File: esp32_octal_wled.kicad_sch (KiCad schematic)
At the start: 54 parts, among them J1 LED1, J11 I2C_Display, J12 ATX-24, J13 LED1, J14 LED1, J15 LED1, J16 LED1, J2 LED1, J3 PROG, J4 LED1, J5 EXT2, J6 LED1, J7 LED1, J8 CPU12V, Q2 BC847, SW1 ON 485 OFF, SW2 RESET, SW4 PROG, U1 AMS1117-3.3, U2 ESP32-WROOM-E, U3 74AHCT125, U4 74AHCT125, U5 MAX3485

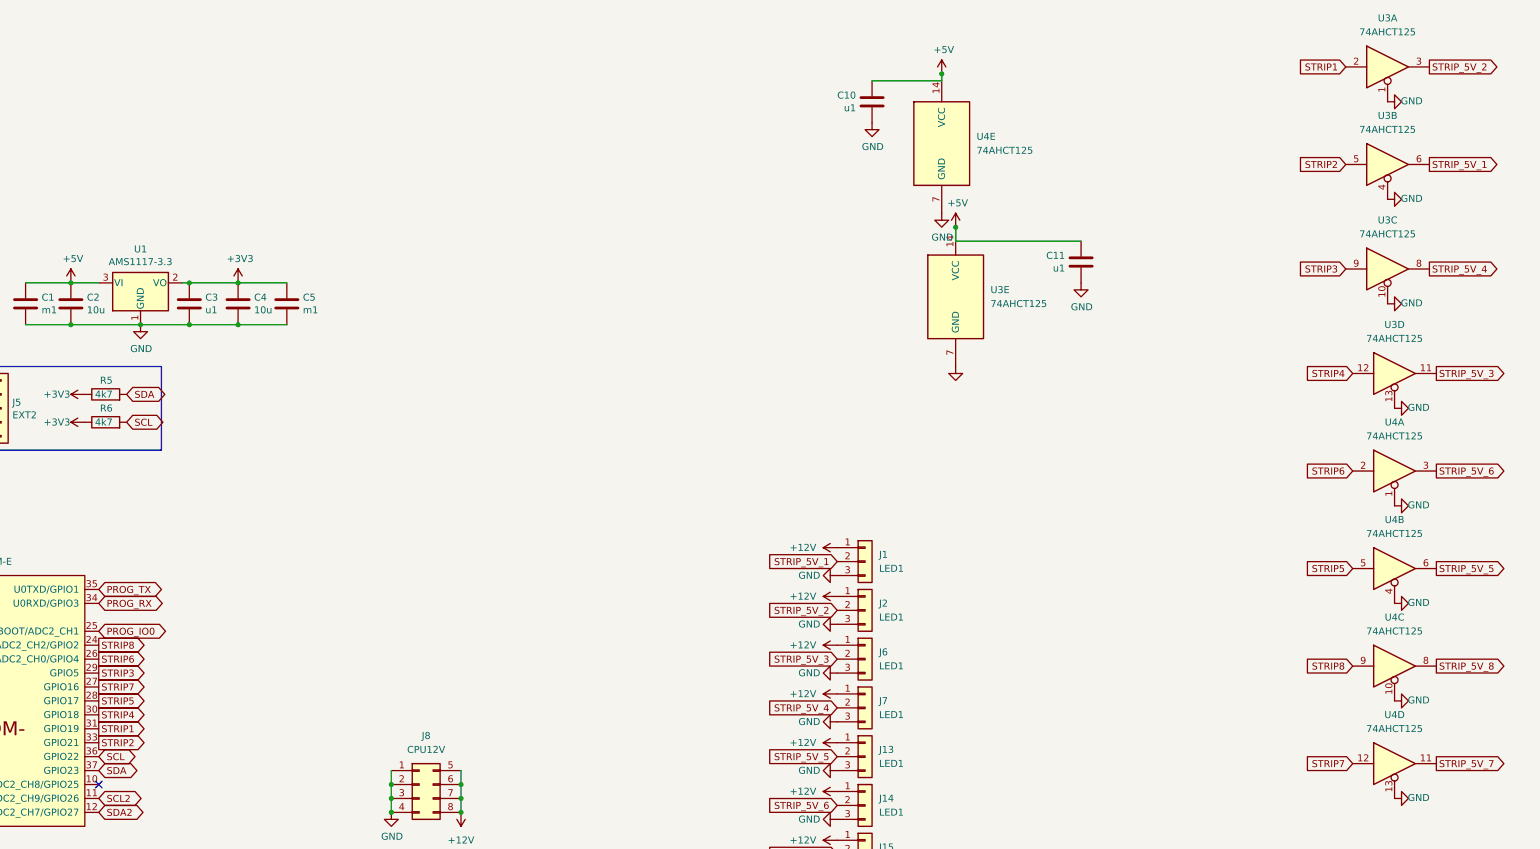
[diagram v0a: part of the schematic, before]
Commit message: Fixes
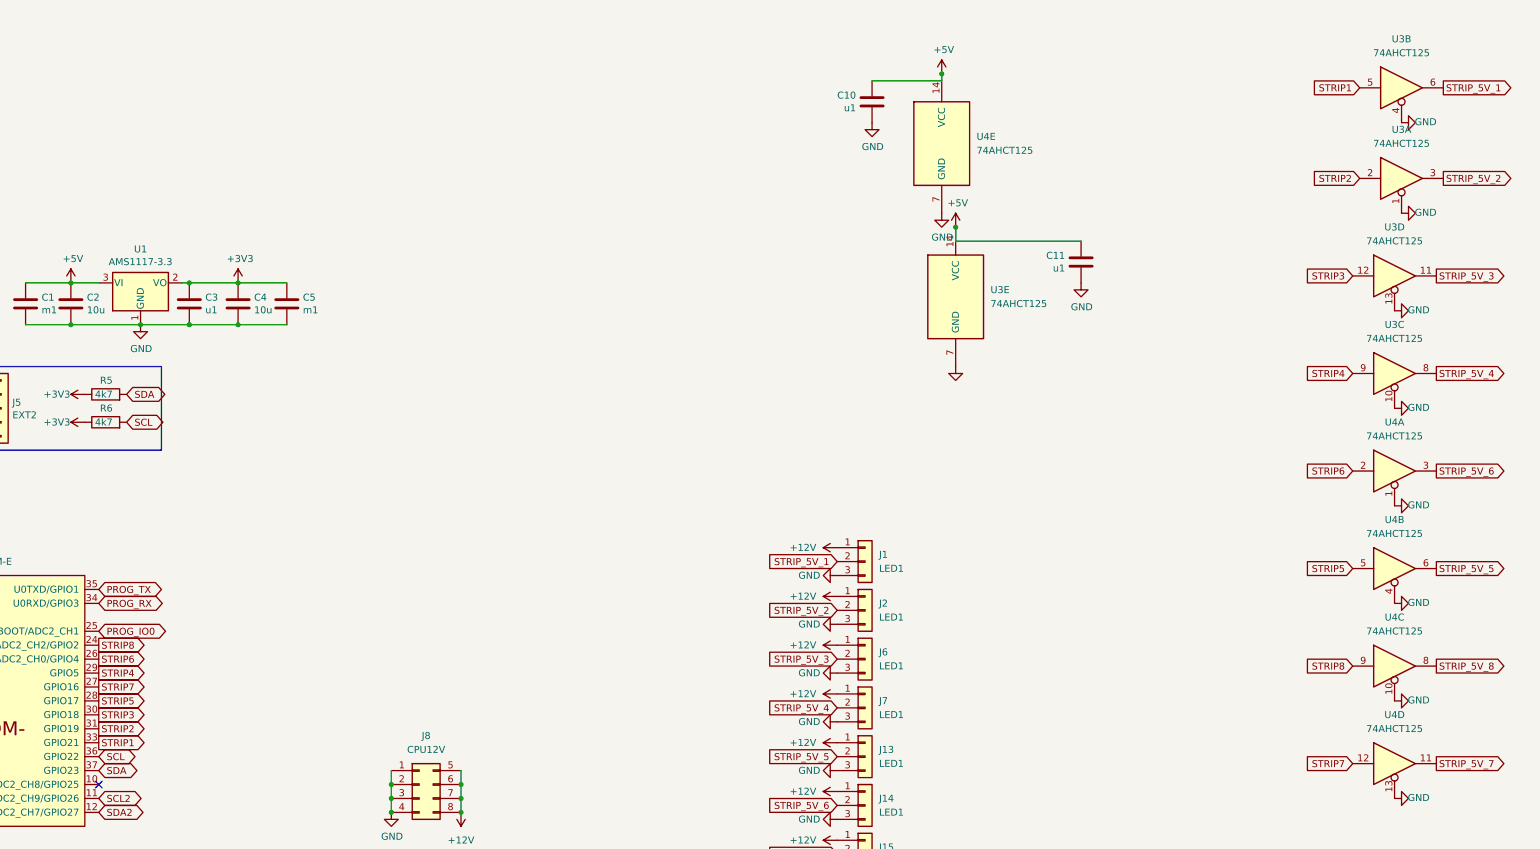
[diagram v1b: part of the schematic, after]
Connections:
- net STRIP1: now also U2.33 (GPIO21), U3.5; no longer U2.31 (GPIO19), U3.2
- net STRIP2: now also U2.31 (GPIO19), U3.2; no longer U2.33 (GPIO21), U3.5
- net STRIP3: now also U2.30 (GPIO18), U3.12; no longer U2.29 (GPIO5), U3.9
- net STRIP4: now also U2.29 (GPIO5), U3.9; no longer U2.30 (GPIO18), U3.12
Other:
- moved on the sheet: U3A, U3B, U3C, U3D

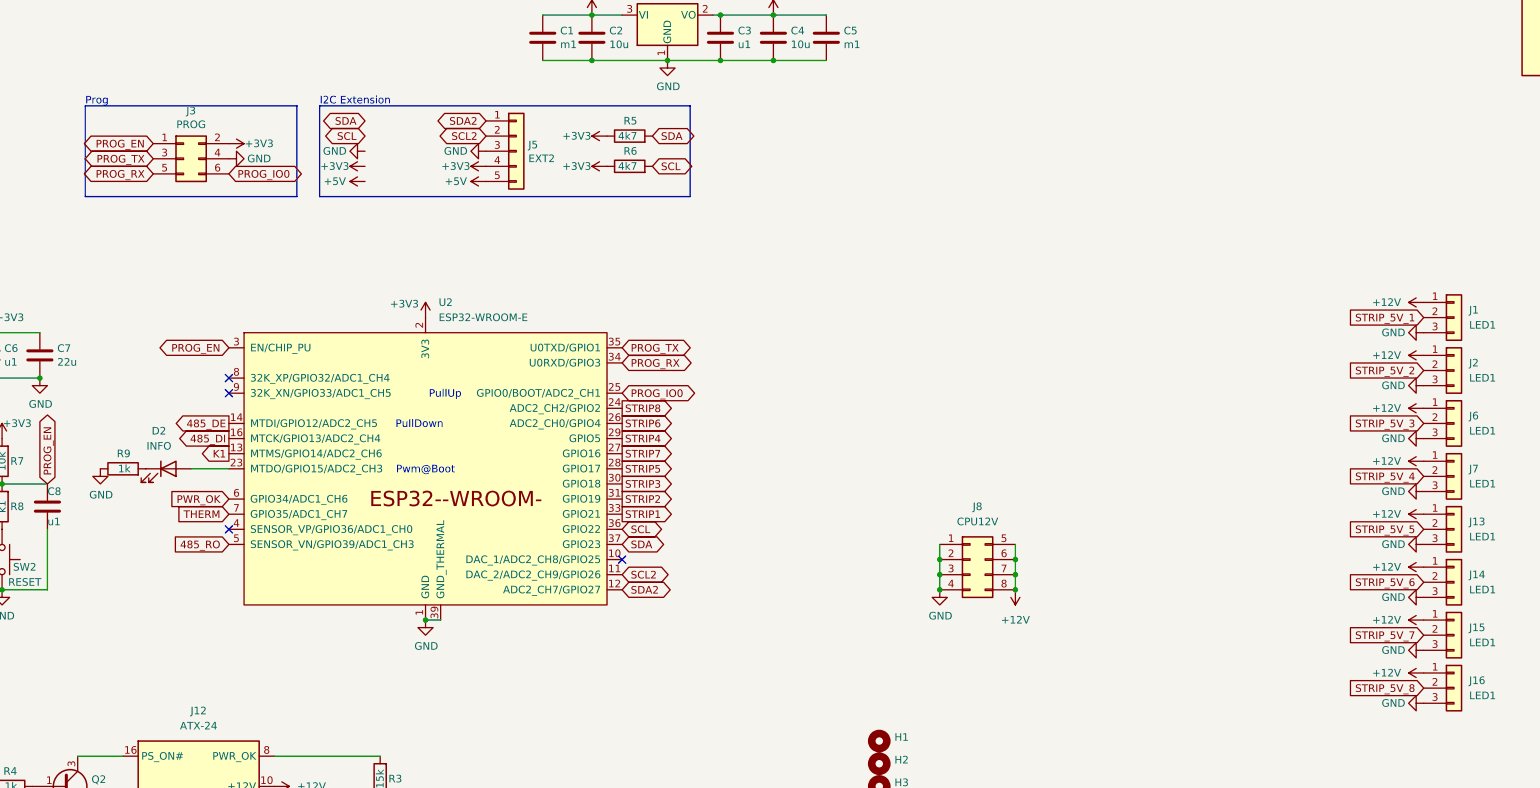
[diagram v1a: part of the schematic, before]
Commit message: INMP441
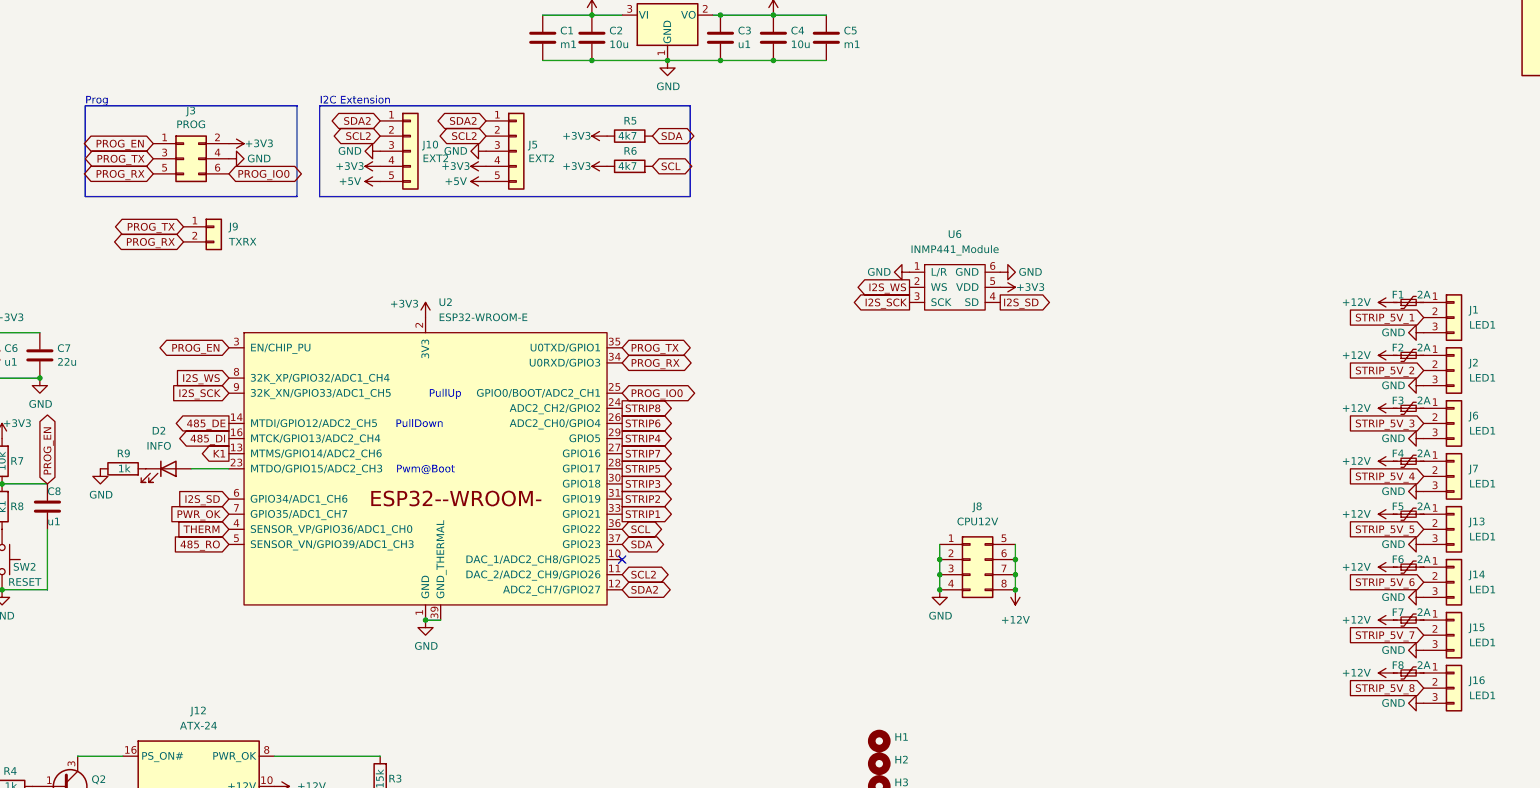
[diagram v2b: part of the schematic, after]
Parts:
- added F1, F2, F3, F4, F5, F6, F7, F8: 2A, Fuse:Fuse_2920_7451Metric_Pad2.10x5.45mm_HandSolder, symbol Device:Polyfuse_Small
- added J10: EXT2, Connector_JST:JST_XH_B5B-XH-A_1x05_P2.50mm_Vertical, symbol Connector_Generic:Conn_01x05
- added J9: TXRX, TestPoint:TestPoint_2Pads_Pitch2.54mm_Drill0.8mm, symbol Connector_Generic:Conn_01x02
- added U6: INMP441_Module, liebler_MODULES:INMP441_Module, symbol smopla:INMP441_Module
- J3: footprint liebler_CONN:IDC_2x03_P1.27mm_Vertical -> Connector:Tag-Connect_TC2030-IDC-NL_2x03_P1.27mm_Vertical
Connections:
- net +12V: now also F1.1, F2.1, F3.1, F4.1, F5.1, F6.1, F7.1, F8.1; no longer J1.1 (Pin_1), J13.1 (Pin_1), J14.1 (Pin_1), J15.1 (Pin_1), J16.1 (Pin_1), J2.1 (Pin_1), J6.1 (Pin_1), J7.1 (Pin_1)
- net +3V3: now also J10.4 (Pin_4), U6.5 (VDD)
- net +5V: now also J10.5 (Pin_5)
- net GND: now also J10.3 (Pin_3), U6.1 (L/R), U6.6 (GND)
- net PROG_RX: now also J9.2 (Pin_2)
- net PROG_TX: now also J9.1 (Pin_1)
- net PWR_OK: now also U2.7 (GPIO35/ADC1_CH7); no longer U2.6 (GPIO34/ADC1_CH6)
- net SCL2: now also J10.2 (Pin_2)
- net SDA2: now also J10.1 (Pin_1)
- net THERM: now also U2.4 (SENSOR_VP/GPIO36/ADC1_CH0); no longer U2.7 (GPIO35/ADC1_CH7)
- net I2S_WS: now reaches U2.8 (32K_XP/GPIO32/ADC1_CH4)
- net I2S_WS: now also U6.2 (WS)
- net I2S_SCK: now reaches U2.9 (32K_XN/GPIO33/ADC1_CH5)
- net I2S_SCK: now also U6.3 (SCK)
- new net: F4.2, J7.1 (Pin_1)
- new net: F8.2, J16.1 (Pin_1)
- new net: F3.2, J6.1 (Pin_1)
- new net: F6.2, J14.1 (Pin_1)
- new net: F1.2, J1.1 (Pin_1)
- new net: F7.2, J15.1 (Pin_1)
- new net: F5.2, J13.1 (Pin_1)
- new net: F2.2, J2.1 (Pin_1)
- new net I2S_SD: U2.6 (GPIO34/ADC1_CH6), U6.4 (SD)
- no-connect marks 8 -> 5

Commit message: Two layer PCB, other PCB format
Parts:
- removed J10, J5: EXT2, Connector_JST:JST_XH_B5B-XH-A_1x05_P2.50mm_Vertical, symbol Connector_Generic:Conn_01x05
- removed R13: 10k, Resistor_SMD:R_0805_2012Metric_Pad1.20x1.40mm_HandSolder, symbol Device:R
- removed TH1: NTC, Capacitor_THT:C_Disc_D3.4mm_W2.1mm_P2.50mm, symbol Device:Thermistor_NTC
- added J17: BH1750 (0x23), Connector_PinSocket_2.54mm:PinSocket_1x05_P2.54mm_Vertical, symbol Connector_Generic:Conn_01x05
- added J18: BME280 (0x76), Connector_PinSocket_2.54mm:PinSocket_1x04_P2.54mm_Vertical, symbol Connector_Generic:Conn_01x04
- J11: value I2C_Display -> I2C EXT; footprint Connector_PinSocket_2.54mm:PinSocket_1x04_P2.54mm_Vertical -> liebler_CONN:JST_XH_S4B-XH-A-1_1x04_P2.50mm_Horizontal_SmallerCourtyard
- SW1: footprint liebler_MECH:Switch_SS12D00 -> liebler_MECH:SW_SPDT_PCM12_handsolder
- SW2, SW4: footprint Button_Switch_THT:SW_PUSH_6mm_H13mm -> liebler_MECH:SW_SPST_TL3342_smaller_handsolder
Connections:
- net SCL2 is gone; now on net STRIP4: U2.11 (DAC_2/ADC2_CH9/GPIO26)
- net SDA2 is gone; now on net STRIP1: U2.12 (ADC2_CH7/GPIO27)
- net +3V3: now also J17.5 (Pin_5), J18.1 (Pin_1)
- net 485_DE: now also U2.10 (DAC_1/ADC2_CH8/GPIO25); no longer U2.14 (MTDI/GPIO12/ADC2_CH5)
- net 485_DI: now also U2.9 (32K_XN/GPIO33/ADC1_CH5); no longer U2.16 (MTCK/GPIO13/ADC2_CH4)
- net 485_RO: now also U2.8 (32K_XP/GPIO32/ADC1_CH4); no longer U2.5 (SENSOR_VN/GPIO39/ADC1_CH3)
- net GND: now also J4.1 (Pin_1), J17.1 (Pin_1), J17.4 (Pin_4), J18.2 (Pin_2); no longer J4.2 (Pin_2)
- net I2S_SCK: now also U2.5 (SENSOR_VN/GPIO39/ADC1_CH3); no longer U2.9 (32K_XN/GPIO33/ADC1_CH5)
- net I2S_WS: now also U2.7 (GPIO35/ADC1_CH7); no longer U2.8 (32K_XP/GPIO32/ADC1_CH4)
- net K1: now also U2.16 (MTCK/GPIO13/ADC2_CH4); no longer U2.13 (MTMS/GPIO14/ADC2_CH6)
- net PWR_OK: now also U2.28 (GPIO17); no longer U2.7 (GPIO35/ADC1_CH7)
- net RS485A: now also D1.2 (K), J4.3 (Pin_3), SW1.1 (A); no longer D1.1 (K), J4.1 (Pin_1), R1.1
- net RS485B: now also D1.1 (K), J4.2 (Pin_2), R1.1; no longer D1.2 (K), J4.3 (Pin_3), SW1.1 (A)
- net SCL: now also J17.3 (Pin_3), J18.3 (Pin_3)
- net SDA: now also J17.2 (Pin_2), J18.4 (Pin_4)
- net STRIP1: now also U3.2; no longer U2.33 (GPIO21), U3.5
- net STRIP2: now also U2.14 (MTDI/GPIO12/ADC2_CH5), U3.12; no longer U2.31 (GPIO19), U3.2
- net STRIP3: now also U2.13 (MTMS/GPIO14/ADC2_CH6), U3.9; no longer U2.30 (GPIO18), U3.12
- net STRIP4: now also U3.5; no longer U2.29 (GPIO5), U3.9
- net STRIP5: now also U2.33 (GPIO21); no longer U2.28 (GPIO17)
- net STRIP6: now also U2.31 (GPIO19); no longer U2.26 (ADC2_CH0/GPIO4)
- net STRIP7: now also U2.30 (GPIO18), U4.9; no longer U2.27 (GPIO16), U4.12
- net STRIP8: now also U2.29 (GPIO5), U4.12; no longer U2.24 (ADC2_CH2/GPIO2), U4.9
- net STRIP_5V_1: now also U3.3; no longer U3.6
- net STRIP_5V_2: now also U3.11; no longer U3.3
- net STRIP_5V_3: now also U3.8; no longer U3.11
- net STRIP_5V_4: now also U3.6; no longer U3.8
- net STRIP_5V_7: now also U4.8; no longer U4.11
- net STRIP_5V_8: now also U4.11; no longer U4.8
- no-connect marks 5 -> 3
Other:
- moved on the sheet: R1, R5, R6, SW1, U3A, U3B, U3C, U3D
